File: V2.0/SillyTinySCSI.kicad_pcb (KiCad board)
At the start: 4 copper layers, 53.5 x 25 mm, 48 parts, among them J1 DB25_Plug, J2 Micro_SD_Card_Det1, U1 74LVT125, U2 74LVT245, U3 74LVT125, U4 74LVT245, U5 TLV75728PDBVR, U6 Pico W

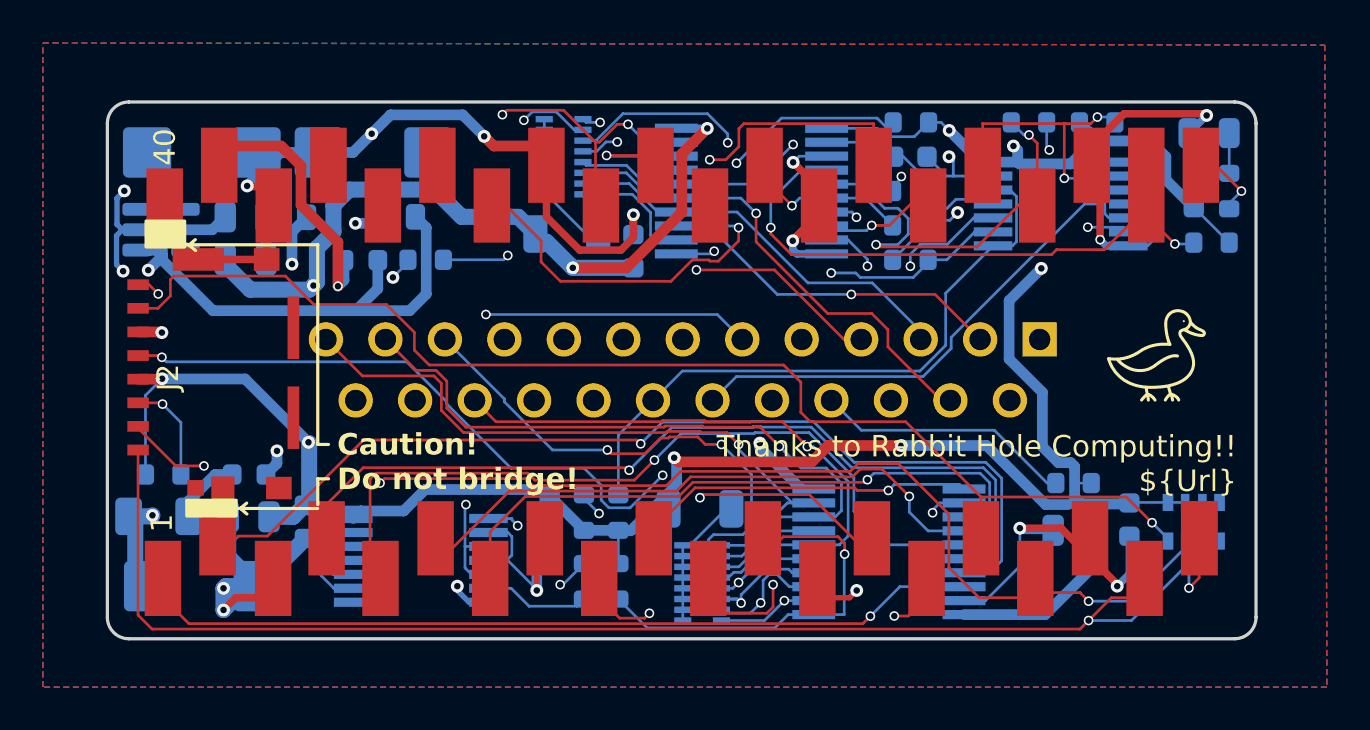
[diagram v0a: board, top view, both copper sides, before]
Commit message: reverted some nuffer changes
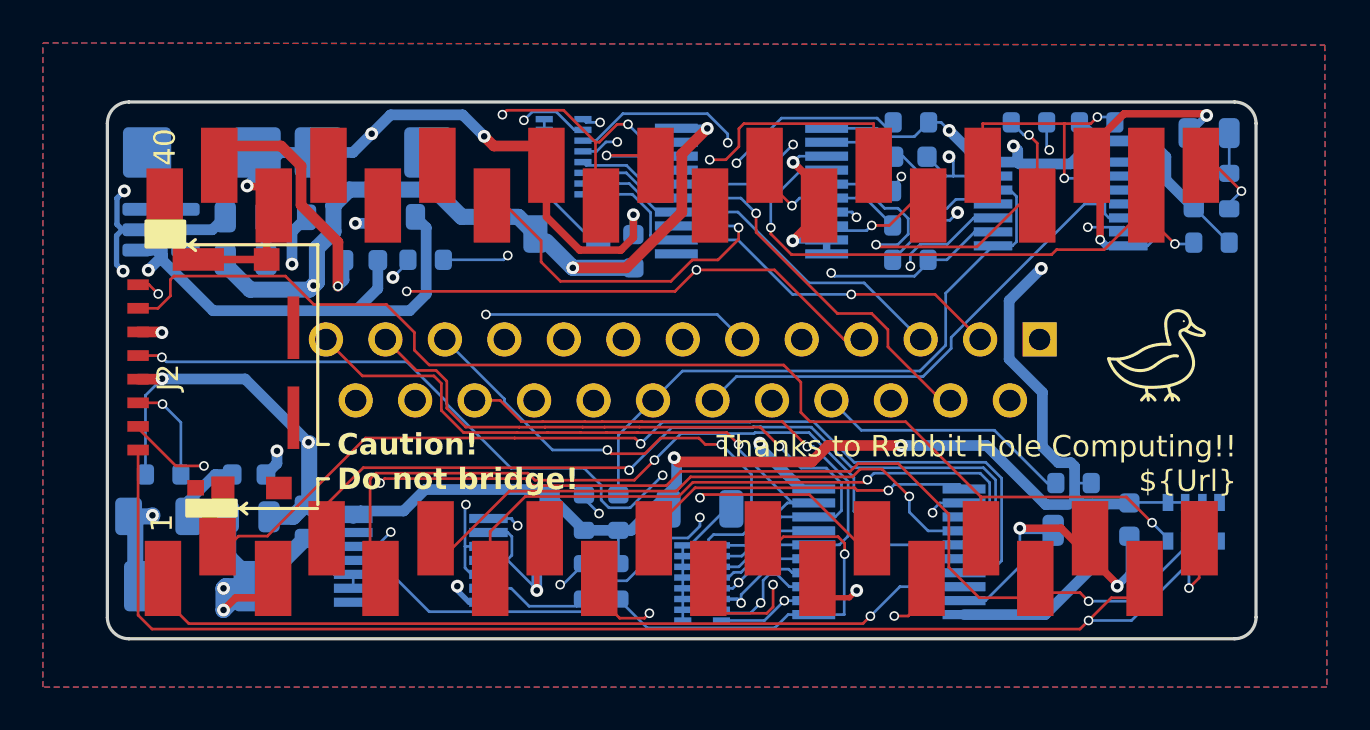
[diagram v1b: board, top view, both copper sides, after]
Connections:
- U1 pad 11: unconnected-(U1-Pad11) -> ~{IN_RST}
- U1 pad 12: GND -> ~{SCSI_RST}
- U2 pad 11: ~{IN_RST} -> unconnected-(U2-B7-Pad11)
- U2 pad 9: ~{SCSI_RST} -> GND
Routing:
- net ~{IN_RST}: track 16.0 -> 47.8 mm
- net ~{SCSI_RST}: track 24.5 -> 45.9 mm, vias 3 -> 4
- net GND: track 134.9 -> 131.8 mm
